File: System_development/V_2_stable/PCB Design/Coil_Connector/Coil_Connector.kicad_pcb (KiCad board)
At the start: 2 copper layers, 16.7 x 22.1 mm, 6 parts, among them J1 Conn_Coaxial

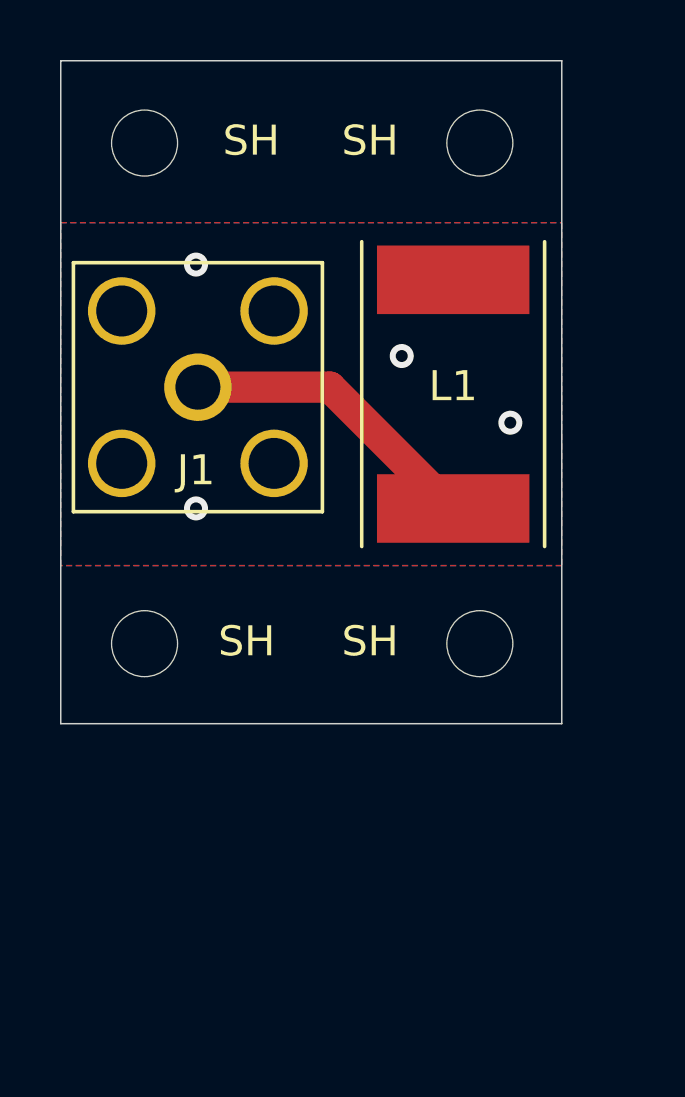
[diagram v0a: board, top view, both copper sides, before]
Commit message: Coil PCB & HP Amp PCB
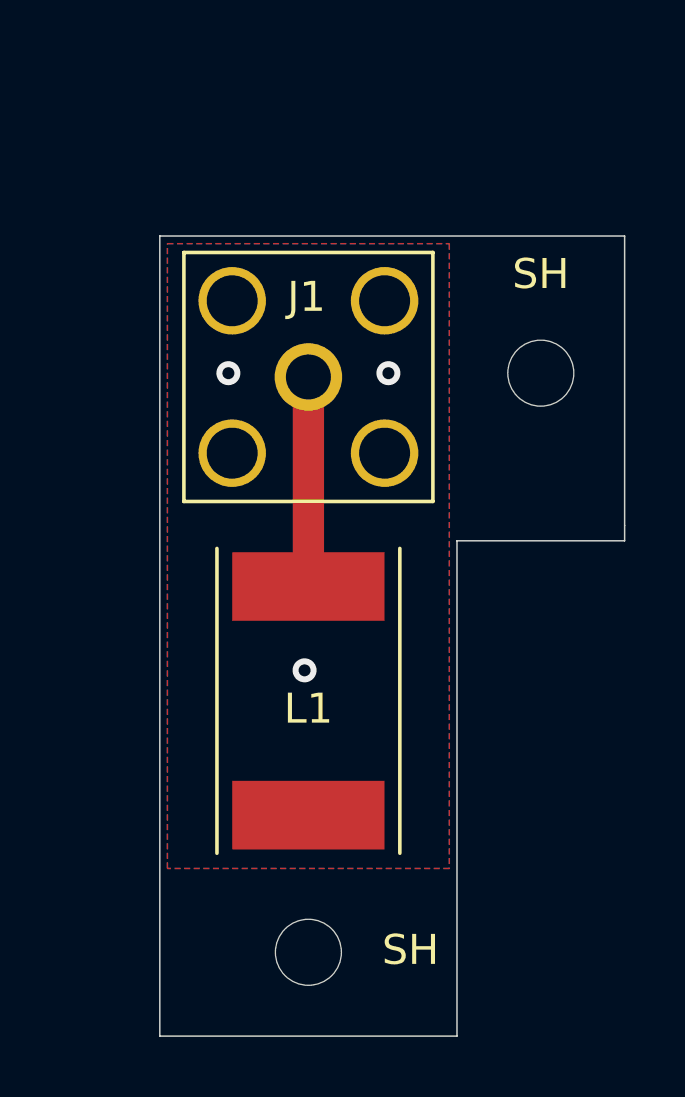
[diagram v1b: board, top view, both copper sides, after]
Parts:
- removed the SH at (144.8, 93.7)
- removed the SH at (144.8, 110.4)
- moved SH 15.3 mm to (146.8, 101.3)
- moved SH 11.6 mm to (139.1, 120.7)
- moved L1 6.69 mm to (139.1, 109.5), turned to 180 degrees
- moved J1 3.70 mm to (139.1, 101.5)
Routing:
- net Net-(J1-Pad1): track 10.2 -> 6.98 mm
- net GND: vias 4 -> 3
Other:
- board size 16.7 x 22.1 mm -> 15.5 x 26.7 mm
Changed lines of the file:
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@@
   (net 2 "Net-(J1-Pad1)")
   (footprint "Connector_Coaxial:SMA_Amphenol_132203-12_Horizontal" (layer "F.Cu")
-    (at 135.382 101.813001)
+    (at 139.065 101.473)
     (descr "https://www.amphenolrf.com/media/downloads/1769/132203-12.pdf")
     (tags "SMA THT Female Jack Horizontal")
     (attr through_hole)
-    (fp_text reference "J1" (at -0.0635 2.771499 180) (layer "F.SilkS")
+    (fp_text reference "J1" (at -0.0635 -2.667 180) (layer "F.SilkS")
       (effects (font (size 1 1) (thickness 0.15)))
     )
@@
   )
   (footprint "L_Coil:L_Coil" (layer "F.Cu")
-    (at 143.891 104.8385)
+    (at 139.065 109.474 180)
     (attr through_hole)
     (fp_text reference "L1" (at 0 -3.056) (layer "F.SilkS")
@@
     (fp_line (start 3.302 2.54) (end -3.302 2.54) (layer "F.CrtYd") (width 0.12))
     (fp_line (start 3.302 -8.128) (end 3.302 2.54) (layer "F.CrtYd") (width 0.12))
-    (pad "1" smd rect locked (at 0 1.016) (size 5.08 2.286) (layers "F.Cu" "F.Paste" "F.Mask")
+    (pad "1" smd rect locked (at 0 1.016 180) (size 5.08 2.286) (layers "F.Cu" "F.Paste" "F.Mask")
       (net 2 "Net-(J1-Pad1)"))
-    (pad "2" smd rect locked (at 0 -6.604) (size 5.08 2.286) (layers "F.Cu" "F.Paste" "F.Mask")
+    (pad "2" smd rect locked (at 0 -6.604 180) (size 5.08 2.286) (layers "F.Cu" "F.Paste" "F.Mask")
       (net 1 "GND"))
   )
   (footprint "MountingHole:MountingHole_2.2mm_M2" (layer "F.Cu")
-    (at 144.78 93.6752)
-    (descr "Mounting Hole 2.2mm, no annular, M2")
-    (tags "mounting hole 2.2mm no annular m2")
-    (attr exclude_from_pos_files exclude_from_bom)
-    (fp_text reference "SH" (at -3.6576 -0.0762) (layer "F.SilkS")
-      (effects (font (size 1 1) (thickness 0.15)))
-    )
-    (fp_text value "MountingHole_2.2mm_M2" (at 0 3.2) (layer "F.Fab")
-      (effects (font (size 1 1) (thickness 0.15)))
-    )
-    (fp_text user "${REFERENCE}" (at 0.3 0) (layer "F.Fab")
-      (effects (font (size 1 1) (thickness 0.15)))
-    )
-    (fp_circle (center 0 0) (end 2.2 0) (layer "Cmts.User") (width 0.15) (fill none))
-    (fp_circle (center 0 0) (end 2.45 0) (layer "F.CrtYd") (width 0.05) (fill none))
-    (pad "" np_thru_hole circle (at 0 0) (size 2.2 2.2) (drill 2.2) (layers *.Cu *.Mask))
-  )
-  (footprint "MountingHole:MountingHole_2.2mm_M2" (layer "F.Cu")
-    (at 133.604 110.363)
+    (at 139.065 120.65)
     (descr "Mounting Hole 2.2mm, no annular, M2")
     (tags "mounting hole 2.2mm no annular m2")
@@
   )
   (footprint "MountingHole:MountingHole_2.2mm_M2" (layer "F.Cu")
-    (at 133.604 93.6752)
+    (at 146.812 101.346)
     (descr "Mounting Hole 2.2mm, no annular, M2")
     (tags "mounting hole 2.2mm no annular m2")
     (attr exclude_from_pos_files exclude_from_bom)
-    (fp_text reference "SH" (at 3.556 -0.0762) (layer "F.SilkS")
+    (fp_text reference "SH" (at 0 -3.302) (layer "F.SilkS")
       (effects (font (size 1 1) (thickness 0.15)))
     )
@@
     (pad "" np_thru_hole circle (at 0 0) (size 2.2 2.2) (drill 2.2) (layers *.Cu *.Mask))
   )
-  (footprint "MountingHole:MountingHole_2.2mm_M2" (layer "F.Cu")
-    (at 144.78 110.363)
-    (descr "Mounting Hole 2.2mm, no annular, M2")
-    (tags "mounting hole 2.2mm no annular m2")
-    (attr exclude_from_pos_files exclude_from_bom)
-    (fp_text reference "SH" (at -3.6576 -0.0762) (layer "F.SilkS")
-      (effects (font (size 1 1) (thickness 0.15)))
-    )
-    (fp_text value "MountingHole_2.2mm_M2" (at 0 3.2) (layer "F.Fab")
-      (effects (font (size 1 1) (thickness 0.15)))
-    )
-    (fp_text user "${REFERENCE}" (at 0.3 0) (layer "F.Fab")
-      (effects (font (size 1 1) (thickness 0.15)))
-    )
-    (fp_circle (center 0 0) (end 2.2 0) (layer "Cmts.User") (width 0.15) (fill none))
-    (fp_circle (center 0 0) (end 2.45 0) (layer "F.CrtYd") (width 0.05) (fill none))
-    (pad "" np_thru_hole circle (at 0 0) (size 2.2 2.2) (drill 2.2) (layers *.Cu *.Mask))
-  )
-  (gr_line (start 147.5105 113.03) (end 147.5105 90.932) (layer "Edge.Cuts") (width 0.05))
-  (gr_line (start 130.81 113.03) (end 147.5105 113.03) (layer "Edge.Cuts") (width 0.05))
-  (gr_line (start 130.81 90.932) (end 130.81 113.03) (layer "Edge.Cuts") (width 0.05))
-  (gr_line (start 147.5105 90.932) (end 130.81 90.932) (layer "Edge.Cuts") (width 0.05))
-  (via (at 145.796 102.997) (size 0.8) (drill 0.4) (layers "F.Cu" "B.Cu") (net 1))
-  (via (at 135.3185 97.7265) (size 0.8) (drill 0.4) (layers "F.Cu" "B.Cu") (net 1))
-  (via (at 135.3185 105.8545) (size 0.8) (drill 0.4) (layers "F.Cu" "B.Cu") (net 1))
-  (via (at 142.1765 100.7745) (size 0.8) (drill 0.4) (layers "F.Cu" "B.Cu") (net 1))
-  (segment (start 139.786001 101.813001) (end 143.891 105.918) (width 1.044) (layer "F.Cu") (net 2))
-  (segment (start 135.382 101.813001) (end 139.786001 101.813001) (width 1.044) (layer "F.Cu") (net 2))
+  (gr_line (start 149.606 96.774) (end 149.606 106.426) (layer "Edge.Cuts") (width 0.05))
+  (gr_line (start 149.606 106.426) (end 149.606 106.934) (layer "Edge.Cuts") (width 0.05))
+  (gr_line (start 144.018 106.934) (end 144.018 123.444) (layer "Edge.Cuts") (width 0.05))
+  (gr_line (start 134.112 96.774) (end 149.606 96.774) (layer "Edge.Cuts") (width 0.05))
+  (gr_line (start 144.018 123.444) (end 134.112 123.444) (layer "Edge.Cuts") (width 0.05))
+  (gr_line (start 149.606 106.934) (end 144.018 106.934) (layer "Edge.Cuts") (width 0.05))
+  (gr_line (start 134.112 123.444) (end 134.112 96.774) (layer "Edge.Cuts") (width 0.05))
+  (via (at 141.732 101.346) (size 0.8) (drill 0.4) (layers "F.Cu" "B.Cu") (free) (net 1))
+  (via (at 136.398 101.346) (size 0.8) (drill 0.4) (layers "F.Cu" "B.Cu") (free) (net 1))
+  (via (at 138.938 111.252) (size 0.8) (drill 0.4) (layers "F.Cu" "B.Cu") (free) (net 1))
+  (segment (start 139.065 101.473) (end 139.065 108.458) (width 1.044) (layer "F.Cu") (net 2))
   (zone (net 1) (net_name "GND") (layer "F.Cu") (hatch edge 0.508)
     (connect_pads (clearance 0.508))
@@
     (polygon
       (pts
-        (xy 147.5105 107.7595)
-        (xy 130.81 107.7595)
-        (xy 130.81 96.3295)
-        (xy 147.5105 96.3295)
+        (xy 143.764 117.856)
+        (xy 134.366 117.856)
+        (xy 134.366 97.028)
+        (xy 143.764 97.028)
       )
     )
@@
     (polygon
       (pts
-        (xy 147.5105 107.7595)
-        (xy 130.81 107.7595)
-        (xy 130.81 96.3295)
-        (xy 147.5105 96.3295)
+        (xy 143.764 117.856)
+        (xy 134.366 117.856)
+        (xy 134.366 97.028)
+        (xy 143.764 97.028)
       )
     )
